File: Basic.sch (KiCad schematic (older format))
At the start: 12 parts, among them J52 Basic, U59 74HC74, U60 74HC02, U61 74HC02, U8 27C010

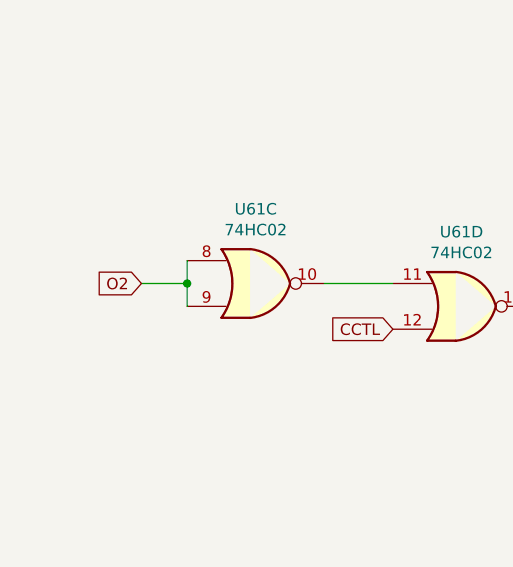
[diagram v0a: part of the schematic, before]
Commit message: Global rebuild up to 1mB
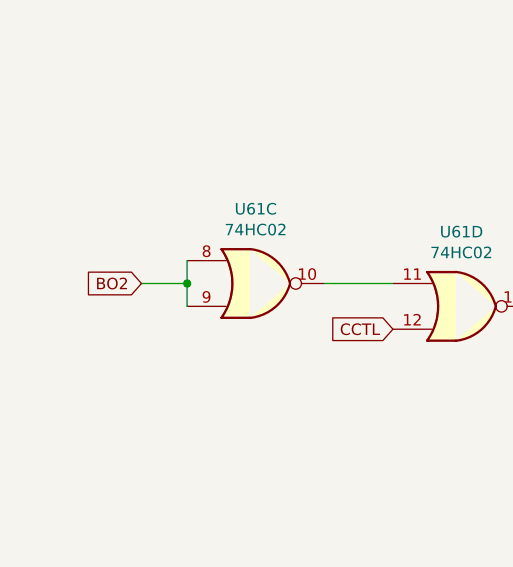
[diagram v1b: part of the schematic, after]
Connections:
- net O2 renamed BO2
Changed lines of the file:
@@
 	1300 3200 1300 3300
 Text GLabel 1100 3300 0    50   Input ~ 0
-O2
+BO2
 Wire Wire Line
 	1100 3300 1300 3300

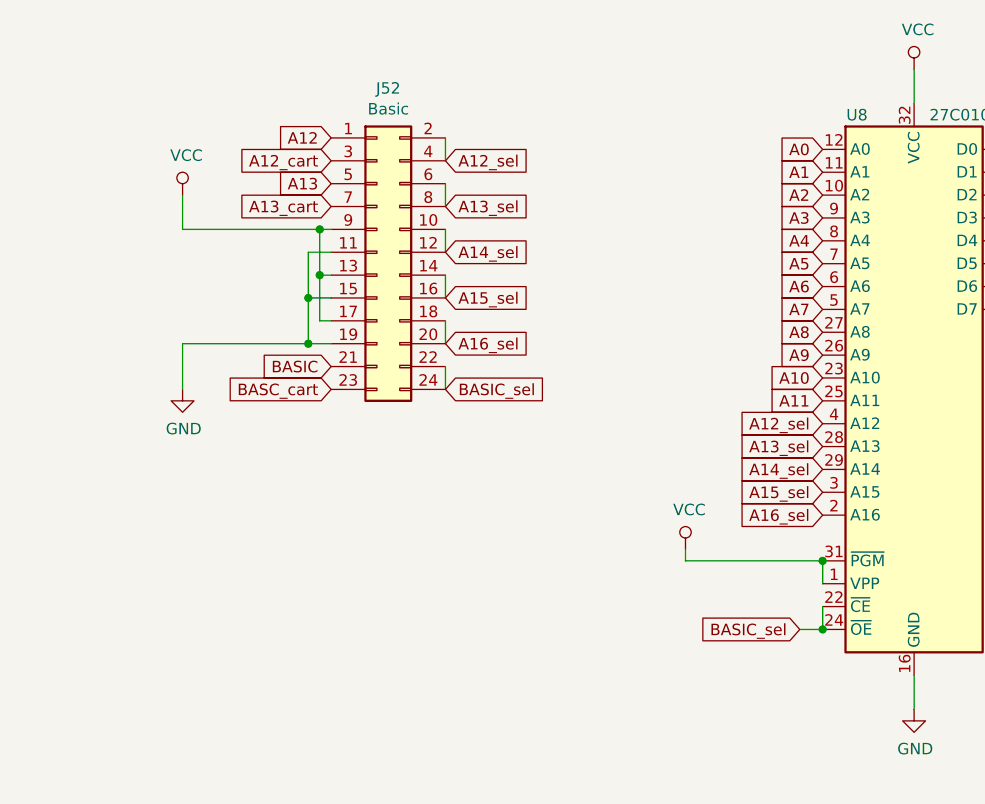
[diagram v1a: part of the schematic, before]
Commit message: Tracking
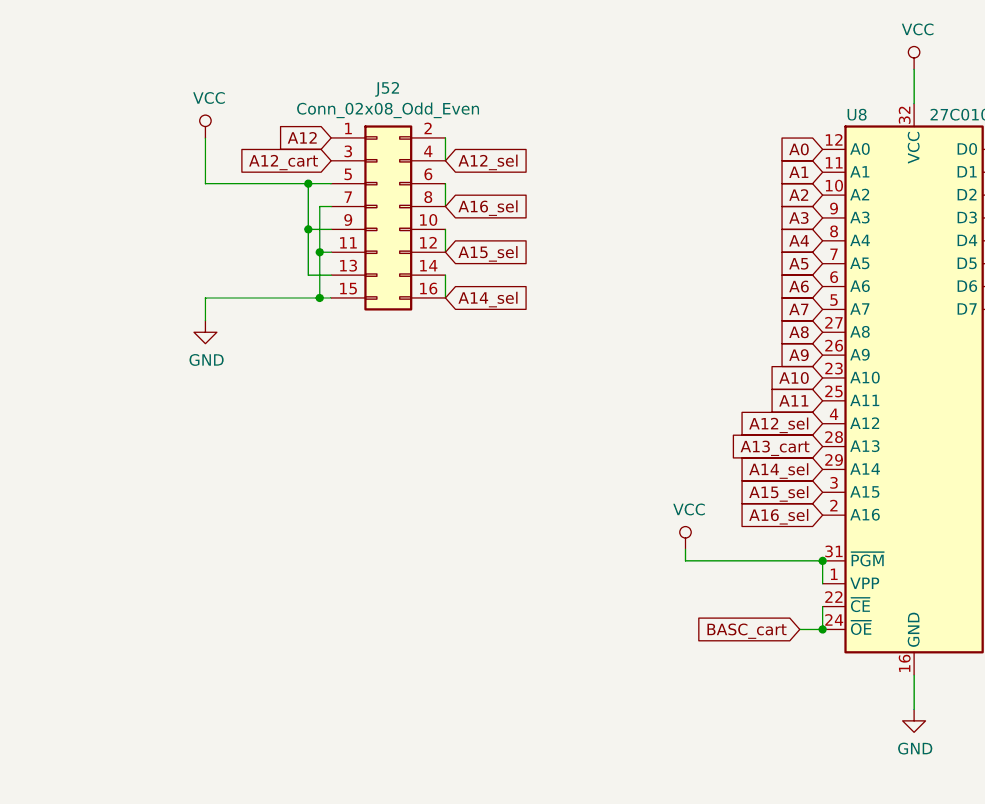
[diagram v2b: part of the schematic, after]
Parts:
- removed J52: Basic, Connector_PinHeader_2.54mm:PinHeader_2x12_P2.54mm_Vertical, symbol Connector_Generic:Conn_02x12_Odd_Even
- added J52: Conn_02x08_Odd_Even, Connector_PinHeader_2.54mm:PinHeader_2x08_P2.54mm_Vertical, symbol Connector_Generic:Conn_02x08_Odd_Even
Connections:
- net A13_sel is gone; now on net A13_cart: U8.28 (A13)
- net BASIC_sel is gone; now on net BASC_cart: U8.22 (~CE), U8.24 (~OE)
- net A12: now also J52.1 (Pin_1)
- net A12_cart: now also J52.3 (Pin_3)
- net A12_sel: now also J52.2 (Pin_2), J52.4 (Pin_4)
- net A14_sel: now also J52.14 (Pin_14), J52.16 (Pin_16)
- net A15_sel: now also J52.10 (Pin_10), J52.12 (Pin_12)
- net A16_sel: now also J52.6 (Pin_6), J52.8 (Pin_8)
- net GND: now also J52.11 (Pin_11), J52.15 (Pin_15), J52.7 (Pin_7)
- net VCC: now also J52.13 (Pin_13), J52.5 (Pin_5), J52.9 (Pin_9)
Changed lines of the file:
@@
 Wire Wire Line
 	9300 3450 9300 3550
-Text GLabel 9200 3550 0    50   Input ~ 0
-BASIC_sel
 Wire Wire Line
 	9200 3550 9300 3550
@@
 Text GLabel 9300 2650 0    50   Input ~ 0
 A12_sel
-Text GLabel 9300 2750 0    50   Input ~ 0
-A13_sel
 Text GLabel 9300 2850 0    50   Input ~ 0
 A14_sel
@@
 Text GLabel 5150 2300 2    50   Input ~ 0
 A13_cart
-Wire Wire Line
-	7650 1400 7650 1500
-Wire Wire Line
-	7650 1600 7650 1700
-Wire Wire Line
-	7650 1800 7650 1900
-Wire Wire Line
-	7650 2000 7650 2100
-Wire Wire Line
-	7650 2200 7650 2300
 Text GLabel 7650 1500 2    50   Input ~ 0
 A12_sel
+Text GLabel 7650 2100 2    50   Input ~ 0
+A14_sel
+Text GLabel 7650 1900 2    50   Input ~ 0
+A15_sel
 Text GLabel 7650 1700 2    50   Input ~ 0
-A13_sel
-Text GLabel 7650 1900 2    50   Input ~ 0
-A14_sel
-Text GLabel 7650 2100 2    50   Input ~ 0
-A15_sel
-Text GLabel 7650 2300 2    50   Input ~ 0
 A16_sel
 Text GLabel 7150 1500 0    50   Input ~ 0
 A12_cart
-Text GLabel 7150 1700 0    50   Input ~ 0
-A13_cart
-Wire Wire Line
-	7150 1800 7100 1800
-Wire Wire Line
-	7100 1800 7100 2000
-Wire Wire Line
-	7100 2000 7150 2000
-Wire Wire Line
-	7100 2000 7100 2200
-Wire Wire Line
-	7100 2200 7150 2200
-Connection ~ 7100 2000
-Wire Wire Line
-	7150 1900 7050 1900
-Wire Wire Line
-	7050 1900 7050 2100
-Wire Wire Line
-	7050 2100 7150 2100
-Wire Wire Line
-	7050 2100 7050 2300
-Wire Wire Line
-	7050 2300 7150 2300
-Connection ~ 7050 2100
-$Comp
-L Connector_Generic:Conn_02x12_Odd_Even J52
-U 1 1 5E6ACC35
-P 7350 1900
-F 0 "J52" H 7400 2617 50  0000 C CNN
-F 1 "Basic" H 7400 2526 50  0000 C CNN
-F 2 "Connector_PinHeader_2.54mm:PinHeader_2x12_P2.54mm_Vertical" H 7350 1900 50  0001 C CNN
-F 3 "~" H 7350 1900 50  0001 C CNN
-	1    7350 1900
-	1    0    0    -1
-$EndComp
-Wire Wire Line
-	7650 2400 7650 2500
-Text GLabel 7650 2500 2    50   Input ~ 0
-BASIC_sel
 Text GLabel 7150 1400 0    50   Input ~ 0
 A12
-Text GLabel 7150 1600 0    50   Input ~ 0
-A13
-Text GLabel 7150 2500 0    50   Input ~ 0
-BASC_cart
-Text GLabel 7150 2400 0    50   Input ~ 0
-BASIC
 Wire Wire Line
 	4850 6475 3900 6475
@@
 L power:VCC #PWR0236
 U 1 1 5E98DD27
-P 6500 1650
-F 0 "#PWR0236" H 6500 1500 50  0001 C CNN
-F 1 "VCC" H 6517 1823 50  0000 C CNN
-F 2 "" H 6500 1650 50  0001 C CNN
-F 3 "" H 6500 1650 50  0001 C CNN
-	1    6500 1650
-	1    0    0    -1
-$EndComp
-Wire Wire Line
-	7100 1800 6500 1800
-Wire Wire Line
-	6500 1800 6500 1650
-Connection ~ 7100 1800
+P 6600 1400
+F 0 "#PWR0236" H 6600 1250 50  0001 C CNN
+F 1 "VCC" H 6617 1573 50  0000 C CNN
+F 2 "" H 6600 1400 50  0001 C CNN
+F 3 "" H 6600 1400 50  0001 C CNN
+	1    6600 1400
+	1    0    0    -1
+$EndComp
 $Comp
 L power:GND #PWR0237
 U 1 1 5E991899
-P 6500 2500
-F 0 "#PWR0237" H 6500 2250 50  0001 C CNN
-F 1 "GND" H 6505 2327 50  0000 C CNN
-F 2 "" H 6500 2500 50  0001 C CNN
-F 3 "" H 6500 2500 50  0001 C CNN
-	1    6500 2500
-	1    0    0    -1
-$EndComp
-Wire Wire Line
-	7050 2300 6500 2300
-Wire Wire Line
-	6500 2300 6500 2500
-Connection ~ 7050 2300
+P 6600 2200
+F 0 "#PWR0237" H 6600 1950 50  0001 C CNN
+F 1 "GND" H 6605 2027 50  0000 C CNN
+F 2 "" H 6600 2200 50  0001 C CNN
+F 3 "" H 6600 2200 50  0001 C CNN
+	1    6600 2200
+	1    0    0    -1
+$EndComp
+Text GLabel 9200 3550 0    50   Input ~ 0
+BASC_cart
+Text GLabel 9300 2750 0    50   Input ~ 0
+A13_cart
+$Comp
+L Connector_Generic:Conn_02x08_Odd_Even J52
+U 1 1 5FA02BA7
+P 7350 1700
+F 0 "J52" H 7400 2217 50  0000 C CNN
+F 1 "Conn_02x08_Odd_Even" H 7400 2126 50  0000 C CNN
+F 2 "Connector_PinHeader_2.54mm:PinHeader_2x08_P2.54mm_Vertical" H 7350 1700 50  0001 C CNN
+F 3 "~" H 7350 1700 50  0001 C CNN
+	1    7350 1700
+	1    0    0    -1
+$EndComp
+Wire Wire Line
+	7650 1400 7650 1500
+Wire Wire Line
+	7650 1600 7650 1700
+Wire Wire Line
+	7650 1800 7650 1900
+Wire Wire Line
+	7650 2000 7650 2100
+Wire Wire Line
+	7150 1600 7050 1600
+Wire Wire Line
+	7050 1600 7050 1800
+Wire Wire Line
+	7050 2000 7150 2000
+Wire Wire Line
+	7150 1800 7050 1800
+Connection ~ 7050 1800
+Wire Wire Line
+	7050 1800 7050 2000
+Wire Wire Line
+	7150 1700 7100 1700
+Wire Wire Line
+	7100 1700 7100 1900
+Wire Wire Line
+	7100 2100 7150 2100
+Wire Wire Line
+	7100 1900 7150 1900
+Connection ~ 7100 1900
+Wire Wire Line
+	7100 1900 7100 2100
+Wire Wire Line
+	6600 1400 6600 1600
+Wire Wire Line
+	6600 1600 7050 1600
+Connection ~ 7050 1600
+Wire Wire Line
+	7100 2100 6600 2100
+Wire Wire Line
+	6600 2100 6600 2200
+Connection ~ 7100 2100
 $EndSCHEMATC

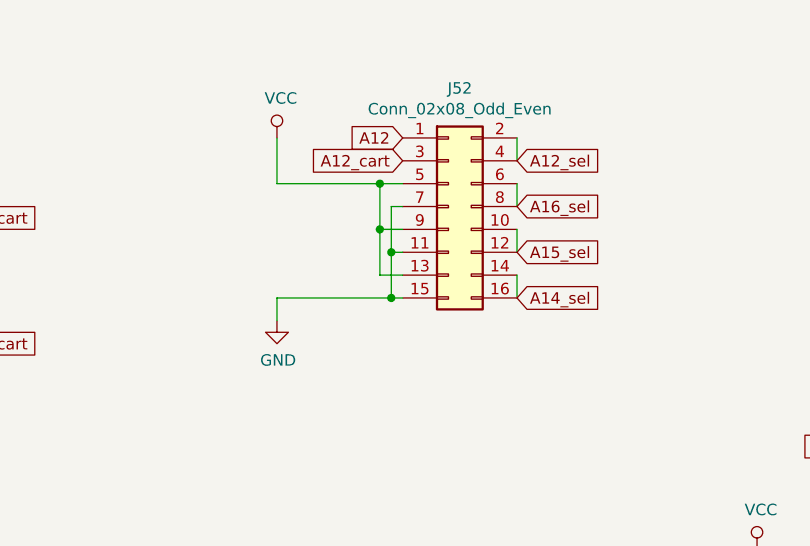
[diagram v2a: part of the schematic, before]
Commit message: Track OS and Basic
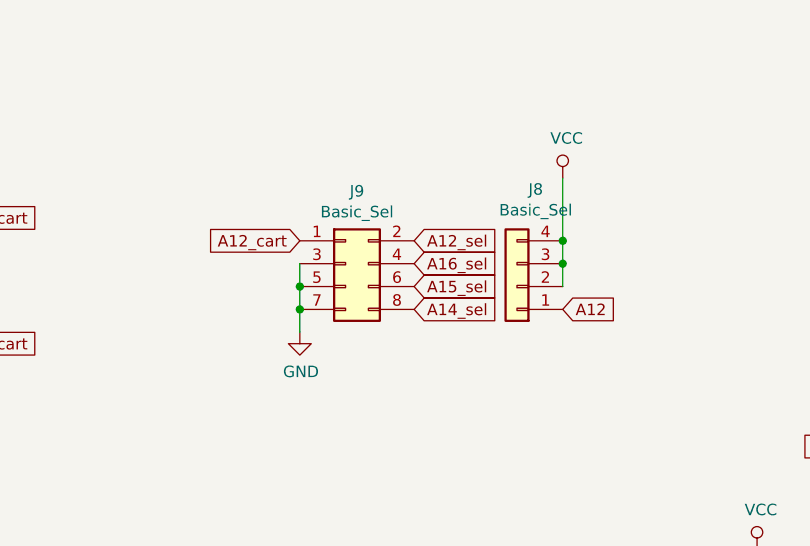
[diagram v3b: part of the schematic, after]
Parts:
- removed J52: Conn_02x08_Odd_Even, Connector_PinHeader_2.54mm:PinHeader_2x08_P2.54mm_Vertical, symbol Connector_Generic:Conn_02x08_Odd_Even
- added J8: Basic_Sel, Connector_PinHeader_2.54mm:PinHeader_1x04_P2.54mm_Vertical, symbol Connector_Generic:Conn_01x04
- added J9: Basic_Sel, Connector_PinHeader_2.54mm:PinHeader_2x04_P2.54mm_Vertical, symbol Connector_Generic:Conn_02x04_Odd_Even
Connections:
- net A12: now also J8.1 (Pin_1)
- net A12_cart: now also J9.1 (Pin_1)
- net A12_sel: now also J9.2 (Pin_2)
- net A14_sel: now also J9.8 (Pin_8)
- net A15_sel: now also J9.6 (Pin_6)
- net A16_sel: now also J9.4 (Pin_4)
- net GND: now also J9.3 (Pin_3), J9.5 (Pin_5), J9.7 (Pin_7)
- net VCC: now also J8.2 (Pin_2), J8.3 (Pin_3), J8.4 (Pin_4)
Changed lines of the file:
@@
 Text GLabel 5150 2300 2    50   Input ~ 0
 A13_cart
-Text GLabel 7650 1500 2    50   Input ~ 0
-A12_sel
-Text GLabel 7650 2100 2    50   Input ~ 0
-A14_sel
-Text GLabel 7650 1900 2    50   Input ~ 0
-A15_sel
-Text GLabel 7650 1700 2    50   Input ~ 0
-A16_sel
-Text GLabel 7150 1500 0    50   Input ~ 0
-A12_cart
-Text GLabel 7150 1400 0    50   Input ~ 0
-A12
 Wire Wire Line
 	4850 6475 3900 6475
@@
 	4550 3900 4550 3400
 Connection ~ 3250 3400
-$Comp
-L power:VCC #PWR0236
-U 1 1 5E98DD27
-P 6600 1400
-F 0 "#PWR0236" H 6600 1250 50  0001 C CNN
-F 1 "VCC" H 6617 1573 50  0000 C CNN
-F 2 "" H 6600 1400 50  0001 C CNN
-F 3 "" H 6600 1400 50  0001 C CNN
-	1    6600 1400
-	1    0    0    -1
-$EndComp
-$Comp
-L power:GND #PWR0237
-U 1 1 5E991899
-P 6600 2200
-F 0 "#PWR0237" H 6600 1950 50  0001 C CNN
-F 1 "GND" H 6605 2027 50  0000 C CNN
-F 2 "" H 6600 2200 50  0001 C CNN
-F 3 "" H 6600 2200 50  0001 C CNN
-	1    6600 2200
-	1    0    0    -1
-$EndComp
 Text GLabel 9200 3550 0    50   Input ~ 0
 BASC_cart
@@
 A13_cart
 $Comp
-L Connector_Generic:Conn_02x08_Odd_Even J52
-U 1 1 5FA02BA7
-P 7350 1700
-F 0 "J52" H 7400 2217 50  0000 C CNN
-F 1 "Conn_02x08_Odd_Even" H 7400 2126 50  0000 C CNN
-F 2 "Connector_PinHeader_2.54mm:PinHeader_2x08_P2.54mm_Vertical" H 7350 1700 50  0001 C CNN
-F 3 "~" H 7350 1700 50  0001 C CNN
-	1    7350 1700
+L Connector_Generic:Conn_01x04 J8
+U 1 1 5FB8A2D8
+P 7650 2050
+F 0 "J8" H 7568 1625 50  0000 C CNN
+F 1 "Basic_Sel" H 7568 1716 50  0000 C CNN
+F 2 "Connector_PinHeader_2.54mm:PinHeader_1x04_P2.54mm_Vertical" H 7650 2050 50  0001 C CNN
+F 3 "~" H 7650 2050 50  0001 C CNN
+	1    7650 2050
+	-1   0    0    1
+$EndComp
+Text GLabel 7200 1850 2    50   Input ~ 0
+A12_sel
+Text GLabel 7200 1950 2    50   Input ~ 0
+A16_sel
+Text GLabel 7200 2050 2    50   Input ~ 0
+A15_sel
+Text GLabel 7200 2150 2    50   Input ~ 0
+A14_sel
+$Comp
+L power:GND #PWR0121
+U 1 1 5FBA1D89
+P 6700 2250
+F 0 "#PWR0121" H 6700 2000 50  0001 C CNN
+F 1 "GND" H 6705 2077 50  0000 C CNN
+F 2 "" H 6700 2250 50  0001 C CNN
+F 3 "" H 6700 2250 50  0001 C CNN
+	1    6700 2250
 	1    0    0    -1
 $EndComp
 Wire Wire Line
-	7650 1400 7650 1500
+	7850 2050 7850 1950
+$Comp
+L power:VCC #PWR0122
+U 1 1 5FBAEFC3
+P 7850 1575
+F 0 "#PWR0122" H 7850 1425 50  0001 C CNN
+F 1 "VCC" H 7867 1748 50  0000 C CNN
+F 2 "" H 7850 1575 50  0001 C CNN
+F 3 "" H 7850 1575 50  0001 C CNN
+	1    7850 1575
+	1    0    0    -1
+$EndComp
+$Comp
+L Connector_Generic:Conn_02x04_Odd_Even J9
+U 1 1 5FBB4F06
+P 6900 1950
+F 0 "J9" H 6950 2267 50  0000 C CNN
+F 1 "Basic_Sel" H 6950 2176 50  0000 C CNN
+F 2 "Connector_PinHeader_2.54mm:PinHeader_2x04_P2.54mm_Vertical" H 6900 1950 50  0001 C CNN
+F 3 "~" H 6900 1950 50  0001 C CNN
+	1    6900 1950
+	1    0    0    -1
+$EndComp
 Wire Wire Line
-	7650 1600 7650 1700
+	6700 2150 6700 2250
 Wire Wire Line
-	7650 1800 7650 1900
+	6700 1950 6700 2050
 Wire Wire Line
-	7650 2000 7650 2100
+	6700 2050 6700 2150
+Connection ~ 6700 2050
+Connection ~ 6700 2150
+Text GLabel 7850 2150 2    50   Input ~ 0
+A12
+Text GLabel 6700 1850 0    50   Input ~ 0
+A12_cart
 Wire Wire Line
-	7150 1600 7050 1600
+	7850 1850 7850 1575
 Wire Wire Line
-	7050 1600 7050 1800
-Wire Wire Line
-	7050 2000 7150 2000
-Wire Wire Line
-	7150 1800 7050 1800
-Connection ~ 7050 1800
-Wire Wire Line
-	7050 1800 7050 2000
-Wire Wire Line
-	7150 1700 7100 1700
-Wire Wire Line
-	7100 1700 7100 1900
-Wire Wire Line
-	7100 2100 7150 2100
-Wire Wire Line
-	7100 1900 7150 1900
-Connection ~ 7100 1900
-Wire Wire Line
-	7100 1900 7100 2100
-Wire Wire Line
-	6600 1400 6600 1600
-Wire Wire Line
-	6600 1600 7050 1600
-Connection ~ 7050 1600
-Wire Wire Line
-	7100 2100 6600 2100
-Wire Wire Line
-	6600 2100 6600 2200
-Connection ~ 7100 2100
+	7850 1950 7850 1850
+Connection ~ 7850 1950
+Connection ~ 7850 1850
 $EndSCHEMATC

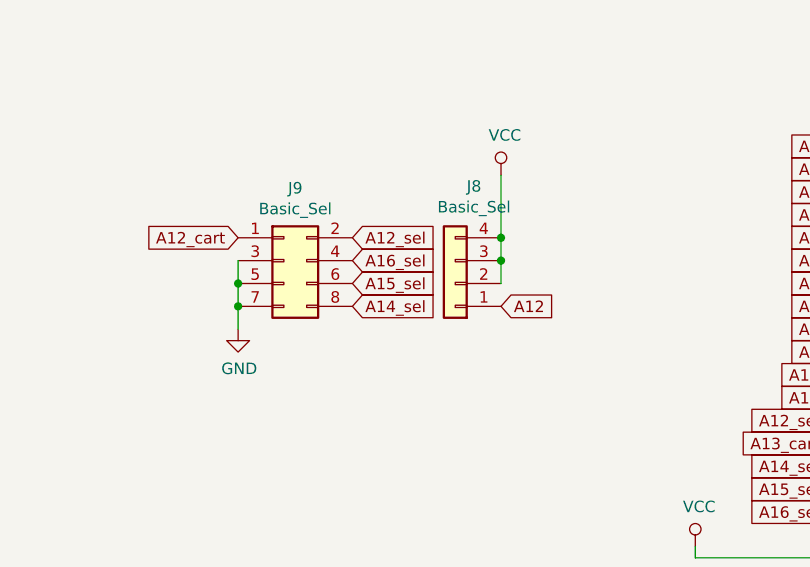
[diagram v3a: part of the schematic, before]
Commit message: Gerber
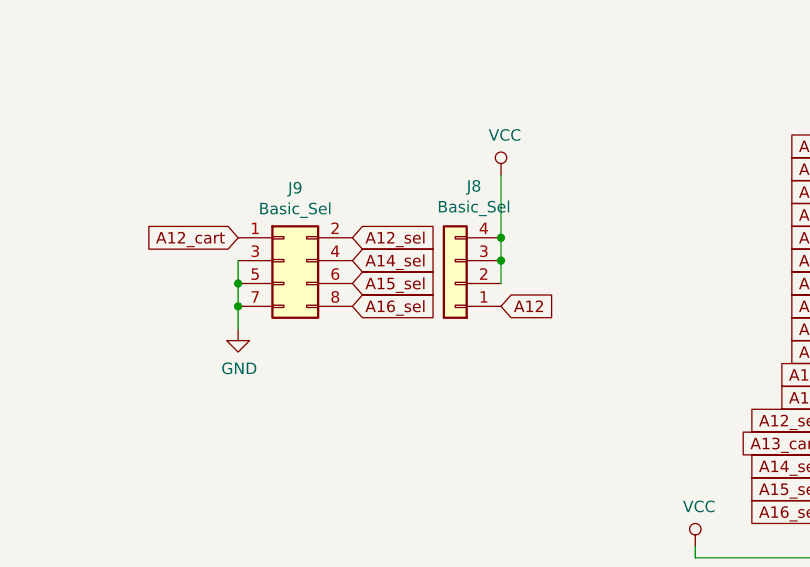
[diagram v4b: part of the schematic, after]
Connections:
- net A14_sel: now also J9.4 (Pin_4); no longer J9.8 (Pin_8)
- net A16_sel: now also J9.8 (Pin_8); no longer J9.4 (Pin_4)
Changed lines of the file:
@@
 Text GLabel 7200 1850 2    50   Input ~ 0
 A12_sel
-Text GLabel 7200 1950 2    50   Input ~ 0
+Text GLabel 7200 2150 2    50   Input ~ 0
 A16_sel
 Text GLabel 7200 2050 2    50   Input ~ 0
 A15_sel
-Text GLabel 7200 2150 2    50   Input ~ 0
+Text GLabel 7200 1950 2    50   Input ~ 0
 A14_sel
 $Comp
